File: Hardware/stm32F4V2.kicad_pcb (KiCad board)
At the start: 2 copper layers, 41.3 x 50.1 mm, 38 parts, among them J1 USB_C_Receptacle_USB2.0_16P, J2 Conn_01x04, J5 Conn_01x18, J6 Conn_01x18, SW1 Push, SW3 Push, U1 STM32F411CCU6, U2 AZ1117-3.3, U4 2SC6, Y2 8MHz

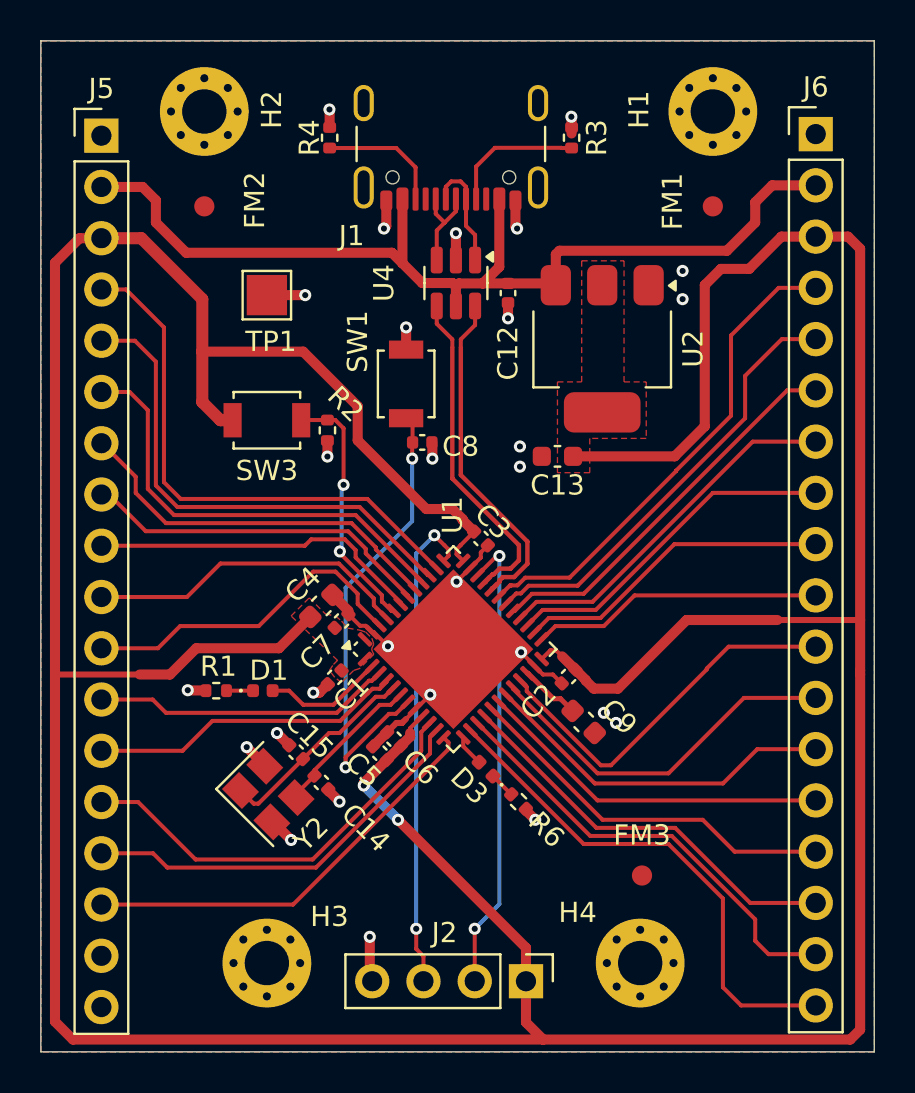
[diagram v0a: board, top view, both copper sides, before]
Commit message: Finalized Layout for V.1
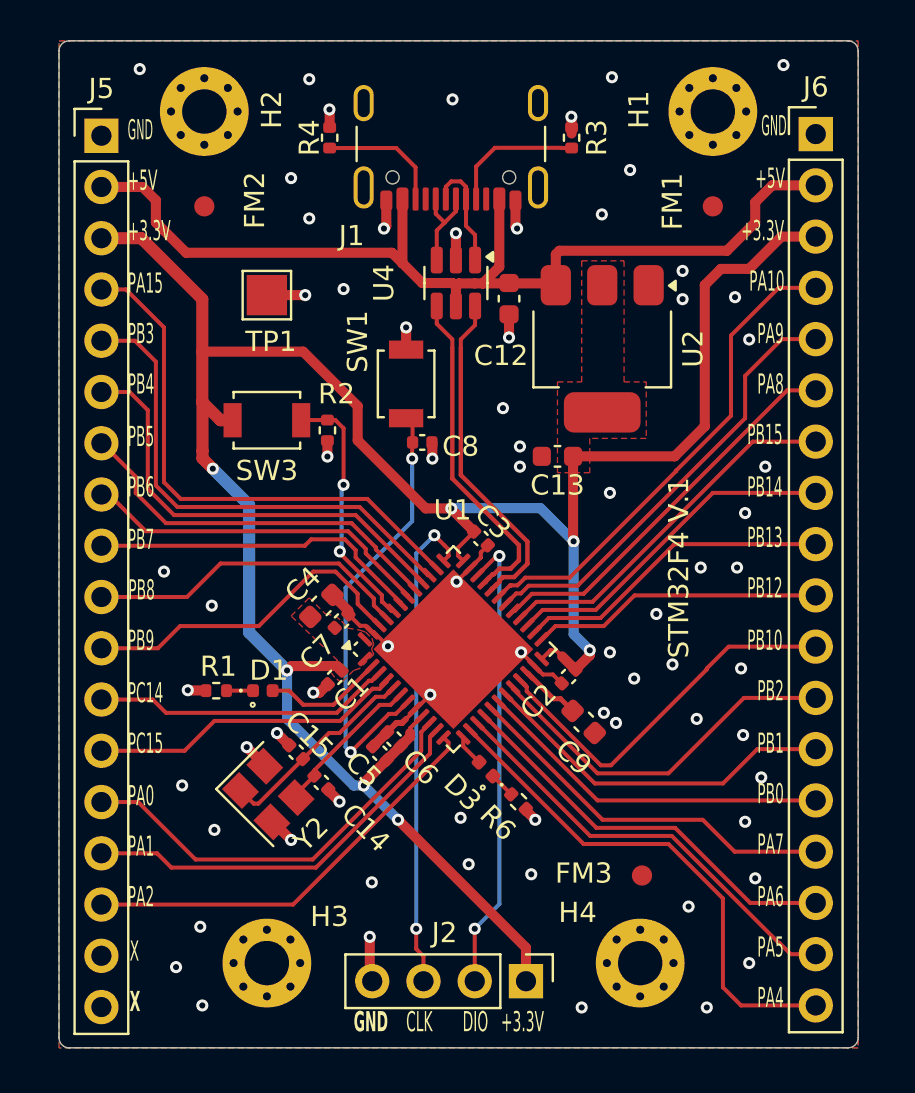
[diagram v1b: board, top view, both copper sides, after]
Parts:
- C12: footprint Capacitor_SMD:C_0402_1005Metric -> Capacitor_SMD:C_0603_1608Metric
- C14, C15: value 10pF -> 10p
- moved C12 0.28 mm to (152.3, 87.3)
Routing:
- net +3.3V: track 229.3 -> 117.5 mm, vias 2 -> 7
- net /NRST: track 23.5 -> 22.0 mm
- net /PA5: track 22.1 -> 21.5 mm
- net GND: track 33.3 -> 33.7 mm, vias 28 -> 71
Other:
- board size 41.3 x 50.1 mm -> 39.6 x 49.9 mm
- board text added: "+3.3V"
- board text added: "+5V"
- board text added: "CLK"
- board text added: "DIO"
- board text added: "GND"
- board text added: "PA0"
- board text added: "PA1"
- board text added: "PA10"
- board text added: "PA15"
- board text added: "PA2"
- board text added: "PA4"
- board text added: "PA5"
- board text added: "PA6"
- board text added: "PA7"
- board text added: "PA8"
- board text added: "PA9"
- board text added: "PB0"
- board text added: "PB1"
- board text added: "PB10"
- board text added: "PB12"
- board text added: "PB13"
- board text added: "PB14"
- board text added: "PB15"
- board text added: "PB2"
- board text added: "PB3"
- board text added: "PB4"
- board text added: "PB5"
- board text added: "PB6"
- board text added: "PB7"
- board text added: "PB8"
- board text added: "PB9"
- board text added: "PC14"
- board text added: "PC15"
- board text added: "STM32F4 V.1"
- board text added: "X"
